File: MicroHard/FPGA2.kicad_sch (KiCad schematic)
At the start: 1 part, among them U4 XC7A100T-FTG256

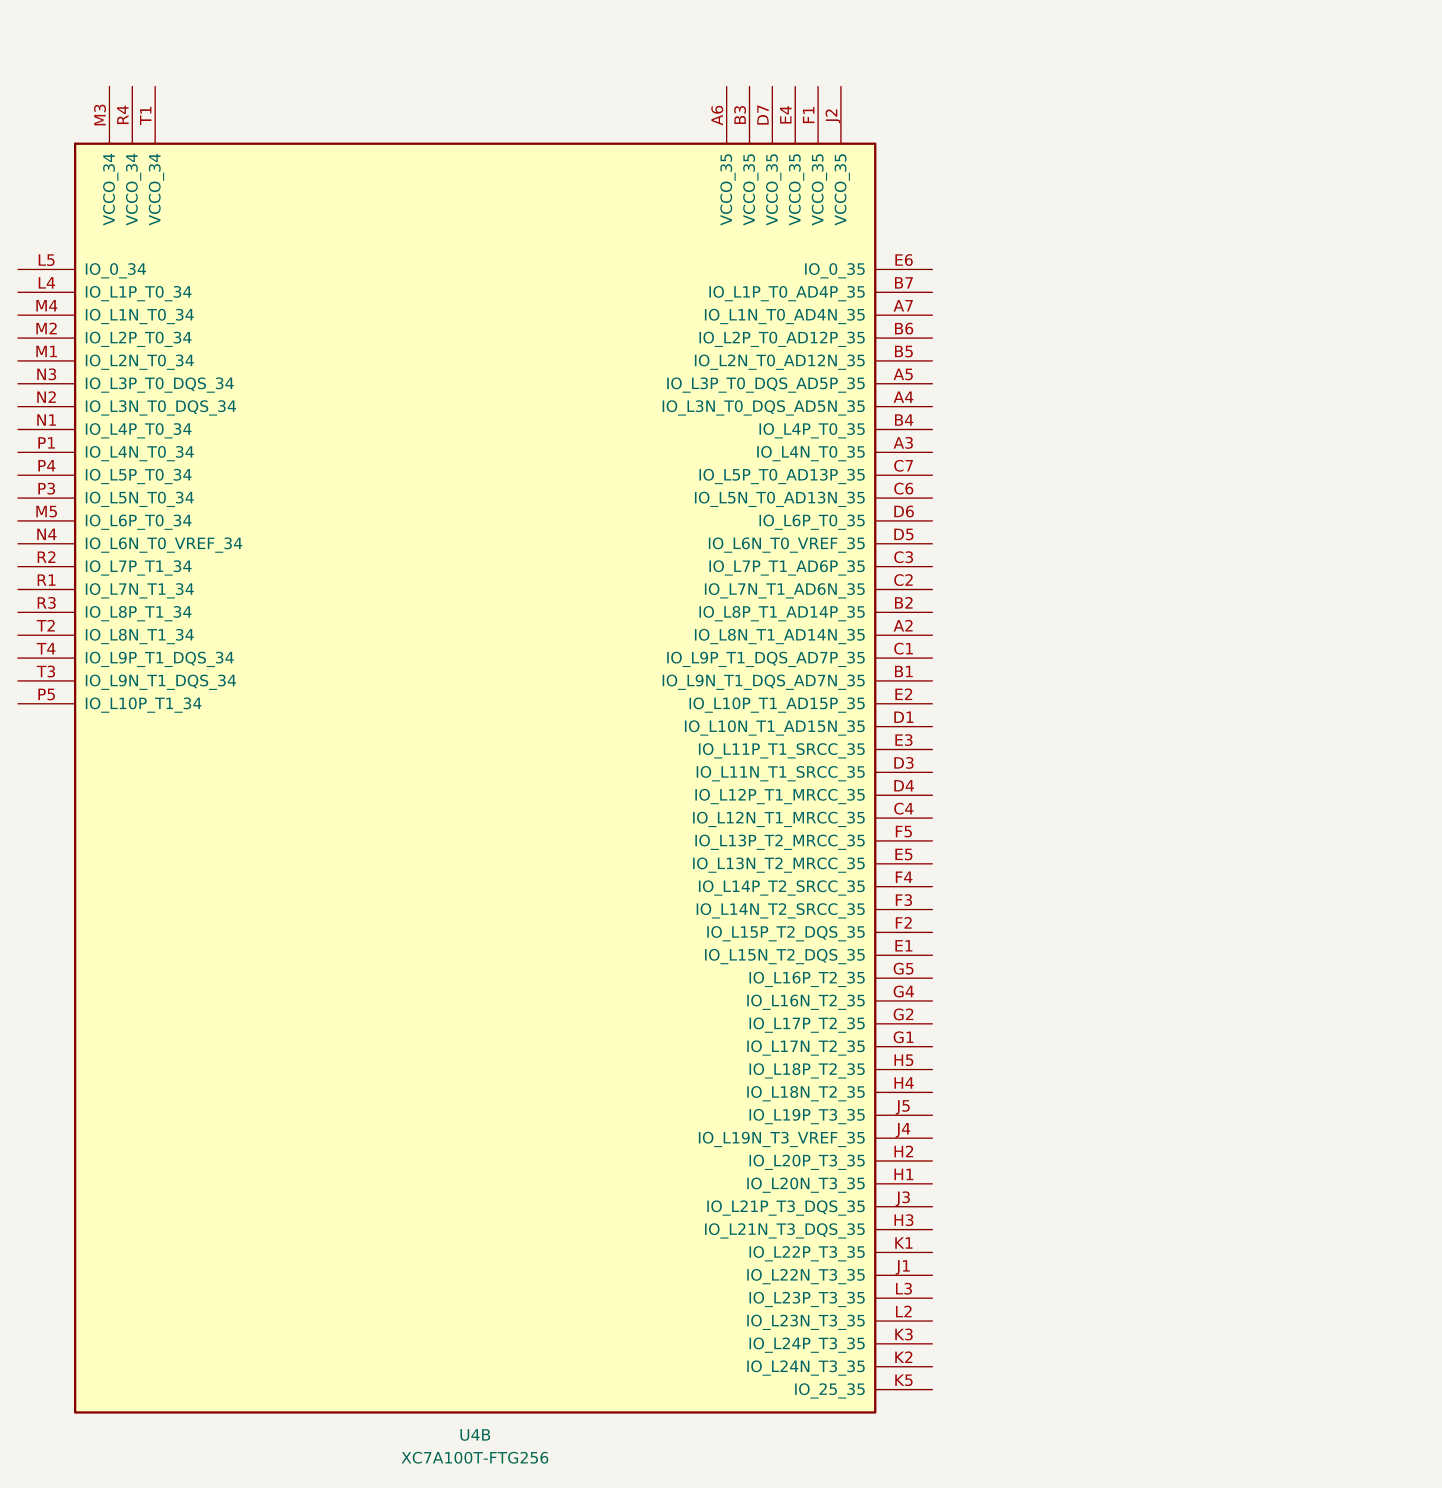
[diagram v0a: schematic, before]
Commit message: feat: finished config
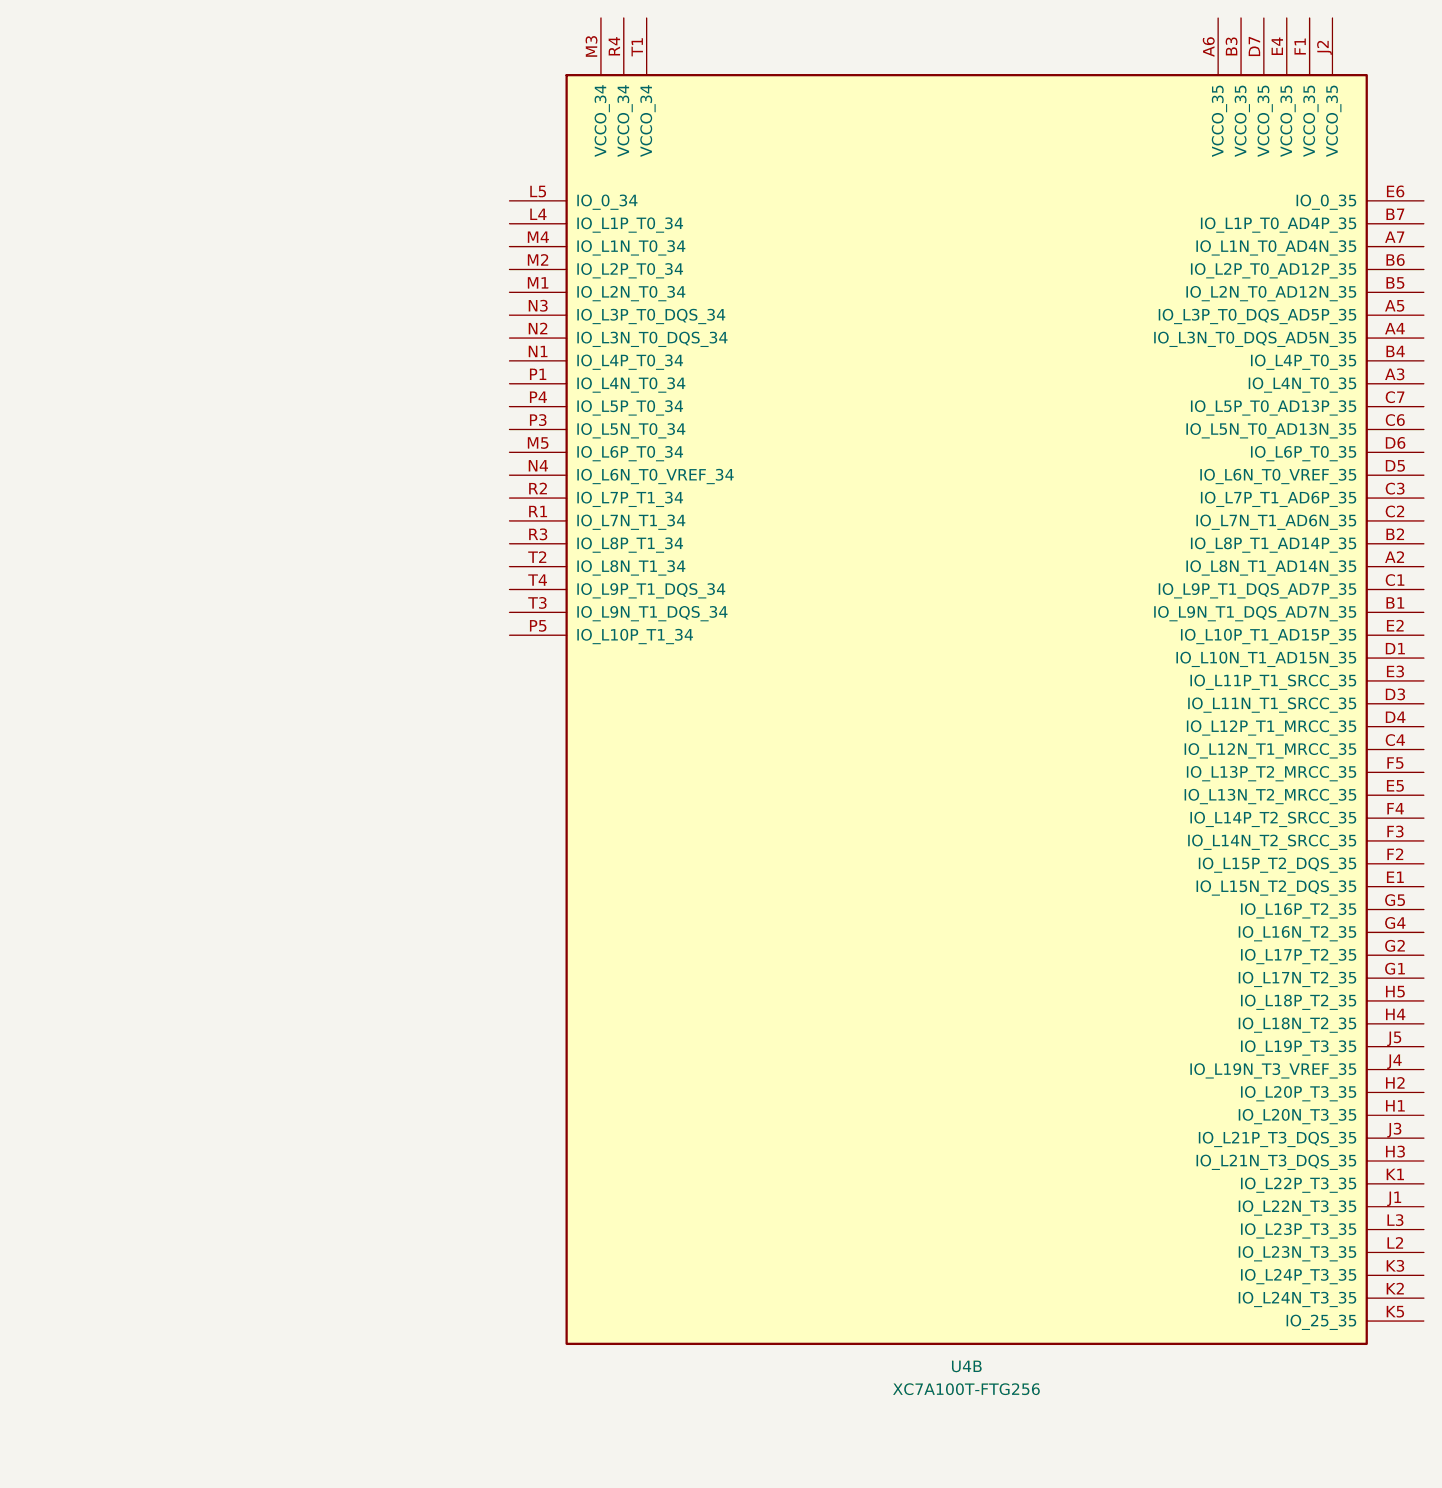
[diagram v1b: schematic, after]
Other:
- moved on the sheet: U4B
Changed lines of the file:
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@@
 	(symbol
 		(lib_id "FPGA_Xilinx_Artix7:XC7A100T-FTG256")
-		(at 87.63 99.06 0)
+		(at 142.24 91.44 0)
 		(unit 2)
 		(exclude_from_sim no)
@@
 		(fields_autoplaced yes)
 		(property "Reference" "U4"
-			(at 87.63 175.26 0)
+			(at 142.24 167.64 0)
 			(effects
 				(font
@@
 		)
 		(property "Value" "XC7A100T-FTG256"
-			(at 87.63 177.8 0)
+			(at 142.24 170.18 0)
 			(effects
 				(font
@@
 		)
 		(property "Footprint" ""
-			(at 87.63 99.06 0)
+			(at 142.24 91.44 0)
 			(effects
 				(font
@@
 		)
 		(property "Datasheet" ""
-			(at 87.63 99.06 0)
+			(at 142.24 91.44 0)
 			(effects
 				(font
@@
 		)
 		(property "Description" "Artix 7 T 100 XC7A100T-FTG256"
-			(at 87.63 99.06 0)
+			(at 142.24 91.44 0)
 			(effects
 				(font
